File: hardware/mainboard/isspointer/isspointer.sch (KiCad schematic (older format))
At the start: 107 parts, among them J1 USB_B_Micro, J2 Motor 1, J3 Motor 2, Q1 SS8050-G, Q2 SS8050-G, Q3 DMN67D8L, Q4 DMN67D8L, SW1 Boot, SW2 Reset, SW3 Up, SW4 Select, SW5 Down, U1 AMS1117-3.3, U2 CP2102N-A01-GQFN28, U3 esp32-WROOM-32D, U4 DRV8834_HTSSOP, U5 DRV8834_HTSSOP, U6 LSM303DLHC, U7 EE-SX3350, U8 EE-SX3350, U9 CFAL12864N

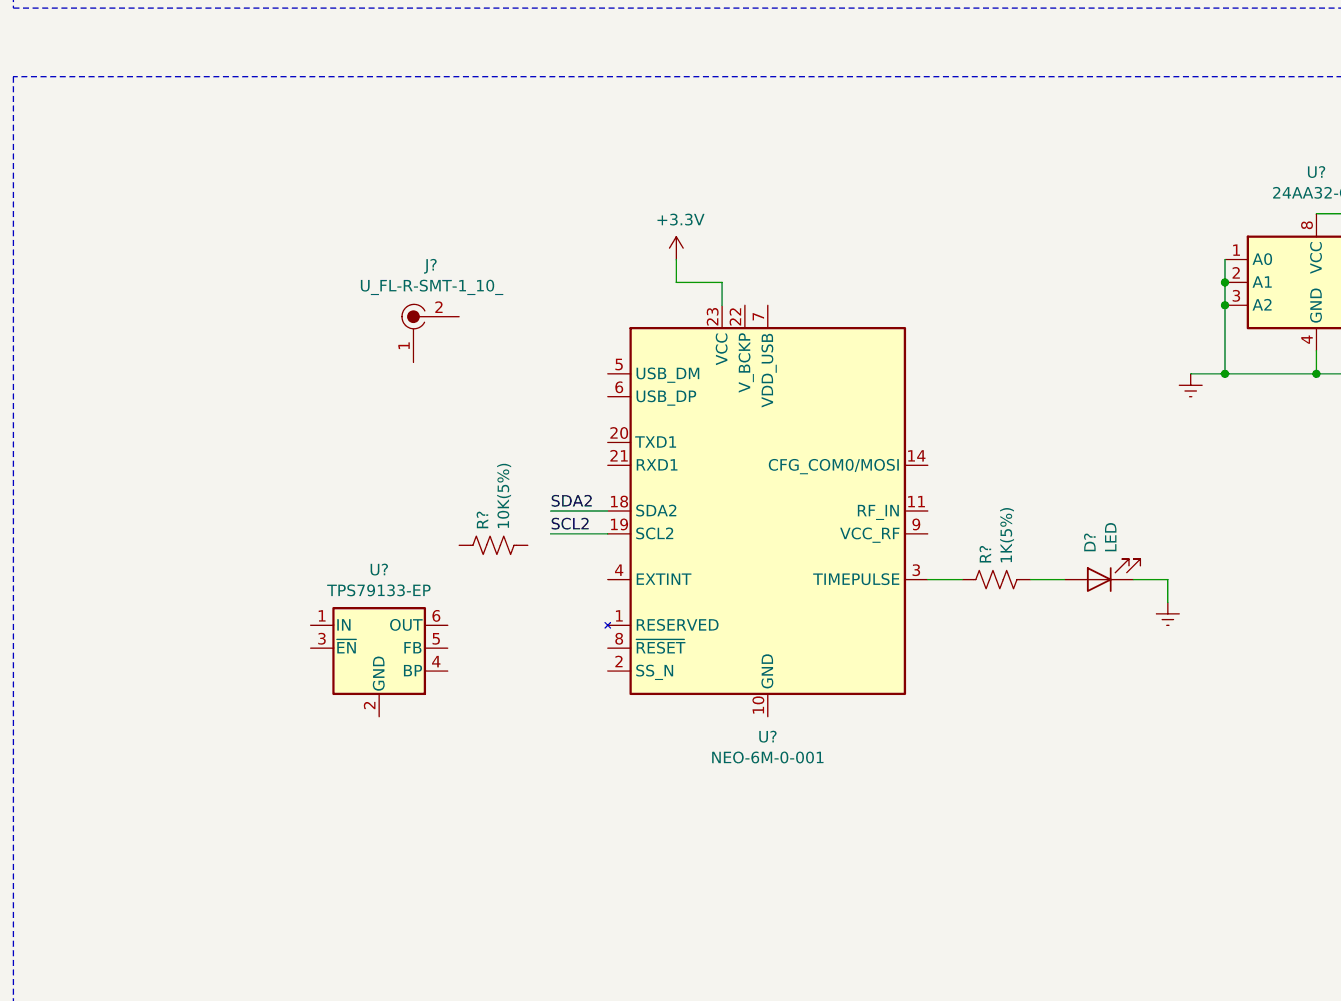
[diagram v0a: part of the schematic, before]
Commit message: minor
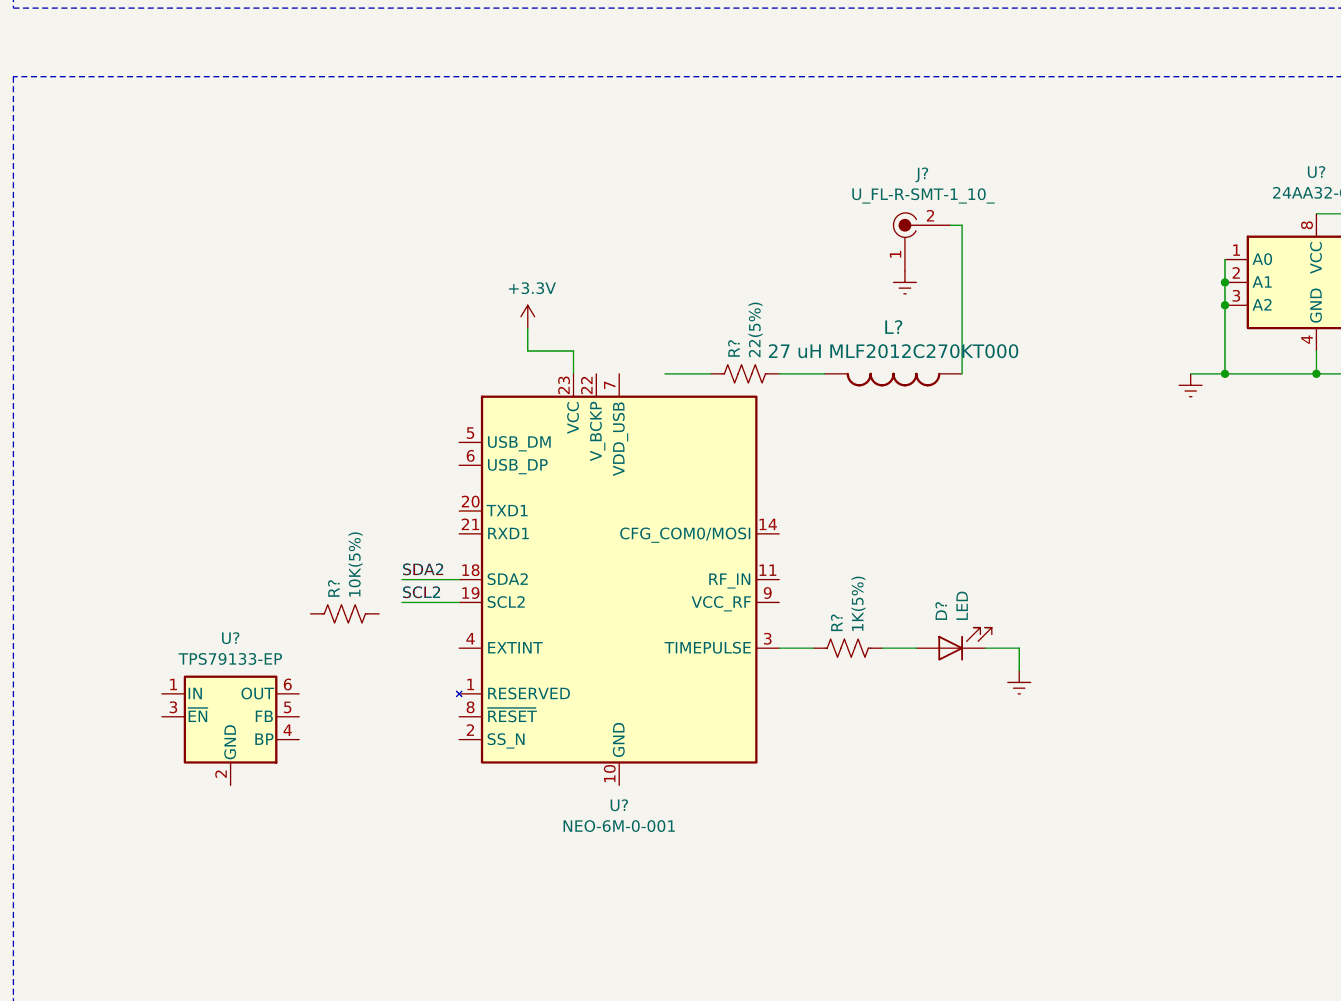
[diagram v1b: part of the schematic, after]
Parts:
- added L?: 27 uH MLF2012C270KT000, symbol isspointer-eagle-import:INDUCTOR0805
- added R?: 22(5%), Resistor_SMD:R_0603_1608Metric_Pad1.05x0.95mm_HandSolder, symbol Device:R_US
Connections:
- net GNDREF: now also J?.1
- net at J?.2: now also L?.1
- new net: L?.2, R?.1
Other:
- moved on the sheet: D?, J?, R?, U?
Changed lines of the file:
@@
 L isspointer:NEO-6M-0-001 U?
 U 1 1 5E5771B3
-P 10650 11800
-F 0 "U?" H 10650 10811 50  0000 C CNN
-F 1 "NEO-6M-0-001" H 10650 10720 50  0000 C CNN
-F 2 "RF_GPS:ublox_NEO" H 11050 10950 50  0001 C CNN
-F 3 "https://www.u-blox.com/sites/default/files/NEO-M8-FW3_DataSheet_%28UBX-15031086%29.pdf" H 10650 11800 50  0001 C CNN
-	1    10650 11800
+P 10000 12100
+F 0 "U?" H 10000 11111 50  0000 C CNN
+F 1 "NEO-6M-0-001" H 10000 11020 50  0000 C CNN
+F 2 "RF_GPS:ublox_NEO" H 10400 11250 50  0001 C CNN
+F 3 "https://www.u-blox.com/sites/default/files/NEO-M8-FW3_DataSheet_%28UBX-15031086%29.pdf" H 10000 12100 50  0001 C CNN
+	1    10000 12100
 	1    0    0    -1
 $EndComp
@@
 L isspointer:TPS79133-EP U?
 U 1 1 5E552781
-P 8950 12400
-F 0 "U?" H 8950 12742 50  0000 C CNN
-F 1 "TPS79133-EP" H 8950 12651 50  0000 C CNN
-F 2 "Package_TO_SOT_SMD:SOT-23-6" H 8950 12725 50  0001 C CIN
-F 3 "http://www.ti.com/lit/ds/symlink/tps79333-ep.pdf" H 8950 12450 50  0001 C CNN
-	1    8950 12400
+P 8300 12700
+F 0 "U?" H 8300 13042 50  0000 C CNN
+F 1 "TPS79133-EP" H 8300 12951 50  0000 C CNN
+F 2 "Package_TO_SOT_SMD:SOT-23-6" H 8300 13025 50  0001 C CIN
+F 3 "http://www.ti.com/lit/ds/symlink/tps79333-ep.pdf" H 8300 12750 50  0001 C CNN
+	1    8300 12700
 	1    0    0    -1
 $EndComp
@@
 	1    0    0    -1
 $EndComp
-Text Label 9700 11800 0    50   ~ 0
+Text Label 9050 12100 0    50   ~ 0
 SDA2
-Text Label 9700 11900 0    50   ~ 0
+Text Label 9050 12200 0    50   ~ 0
 SCL2
 Wire Wire Line
-	9950 11800 9700 11800
-Wire Wire Line
-	9950 11900 9700 11900
+	9300 12100 9050 12100
+Wire Wire Line
+	9300 12200 9050 12200
 Text Label 13700 10700 2    50   ~ 0
 SDA2
@@
 L dk_Coaxial-Connectors-RF:U_FL-R-SMT-1_10_ J?
 U 1 1 5E7CAB51
-P 9100 10950
-F 0 "J?" H 9178 11175 50  0000 C CNN
-F 1 "U_FL-R-SMT-1_10_" H 9178 11084 50  0000 C CNN
-F 2 "digikey-footprints:Coax_Conn_U.FL" H 9300 11150 60  0001 L CNN
-F 3 "https://www.hirose.com/product/en/download_file/key_name/U.FL-R-SMT-1%2810%29/category/Drawing%20(2D)/doc_file_id/37627/?file_category_id=6&item_id=03310472210&is_series=U.FL-R-SMT-1(10" H 9300 11250 60  0001 L CNN
-F 4 "H11891CT-ND" H 9300 11350 60  0001 L CNN "Digi-Key_PN"
-F 5 "U.FL-R-SMT-1(10)" H 9300 11450 60  0001 L CNN "MPN"
-F 6 "Connectors, Interconnects" H 9300 11550 60  0001 L CNN "Category"
-F 7 "Coaxial Connectors (RF)" H 9300 11650 60  0001 L CNN "Family"
-F 8 "https://www.hirose.com/product/en/download_file/key_name/U.FL-R-SMT-1%2810%29/category/Drawing%20(2D)/doc_file_id/37627/?file_category_id=6&item_id=03310472210&is_series=U.FL-R-SMT-1(10" H 9300 11750 60  0001 L CNN "DK_Datasheet_Link"
-F 9 "/product-detail/en/hirose-electric-co-ltd/U.FL-R-SMT-1(10)/H11891CT-ND/2504612" H 9300 11850 60  0001 L CNN "DK_Detail_Page"
-F 10 "CONN U.FL RCPT STR 50 OHM SMD" H 9300 11950 60  0001 L CNN "Description"
-F 11 "Hirose Electric Co Ltd" H 9300 12050 60  0001 L CNN "Manufacturer"
-F 12 "Active" H 9300 12150 60  0001 L CNN "Status"
-	1    9100 10950
+P 11250 10550
+F 0 "J?" H 11328 10775 50  0000 C CNN
+F 1 "U_FL-R-SMT-1_10_" H 11328 10684 50  0000 C CNN
+F 2 "digikey-footprints:Coax_Conn_U.FL" H 11450 10750 60  0001 L CNN
+F 3 "https://www.hirose.com/product/en/download_file/key_name/U.FL-R-SMT-1%2810%29/category/Drawing%20(2D)/doc_file_id/37627/?file_category_id=6&item_id=03310472210&is_series=U.FL-R-SMT-1(10" H 11450 10850 60  0001 L CNN
+F 4 "H11891CT-ND" H 11450 10950 60  0001 L CNN "Digi-Key_PN"
+F 5 "U.FL-R-SMT-1(10)" H 11450 11050 60  0001 L CNN "MPN"
+F 6 "Connectors, Interconnects" H 11450 11150 60  0001 L CNN "Category"
+F 7 "Coaxial Connectors (RF)" H 11450 11250 60  0001 L CNN "Family"
+F 8 "https://www.hirose.com/product/en/download_file/key_name/U.FL-R-SMT-1%2810%29/category/Drawing%20(2D)/doc_file_id/37627/?file_category_id=6&item_id=03310472210&is_series=U.FL-R-SMT-1(10" H 11450 11350 60  0001 L CNN "DK_Datasheet_Link"
+F 9 "/product-detail/en/hirose-electric-co-ltd/U.FL-R-SMT-1(10)/H11891CT-ND/2504612" H 11450 11450 60  0001 L CNN "DK_Detail_Page"
+F 10 "CONN U.FL RCPT STR 50 OHM SMD" H 11450 11550 60  0001 L CNN "Description"
+F 11 "Hirose Electric Co Ltd" H 11450 11650 60  0001 L CNN "Manufacturer"
+F 12 "Active" H 11450 11750 60  0001 L CNN "Status"
+	1    11250 10550
 	1    0    0    -1
 $EndComp
@@
 L Device:R_US R?
 U 1 1 5E7CC5CF
-P 9450 11950
-F 0 "R?" H 9382 11904 50  0000 R CNN
-F 1 "10K(5%)" H 9382 11995 50  0000 R CNN
-F 2 "Resistor_SMD:R_0603_1608Metric_Pad1.05x0.95mm_HandSolder" V 9490 11940 50  0001 C CNN
-F 3 "~" H 9450 11950 50  0001 C CNN
-	1    9450 11950
+P 8800 12250
+F 0 "R?" H 8732 12204 50  0000 R CNN
+F 1 "10K(5%)" H 8732 12295 50  0000 R CNN
+F 2 "Resistor_SMD:R_0603_1608Metric_Pad1.05x0.95mm_HandSolder" V 8840 12240 50  0001 C CNN
+F 3 "~" H 8800 12250 50  0001 C CNN
+	1    8800 12250
 	0    1    1    0
 $EndComp
@@
 L power:+3.3V #PWR?
 U 1 1 5E7F5B7C
-P 10250 10700
-F 0 "#PWR?" H 10250 10550 50  0001 C CNN
-F 1 "+3.3V" H 10267 10873 50  0000 C CNN
-F 2 "" H 10250 10700 50  0001 C CNN
-F 3 "" H 10250 10700 50  0001 C CNN
-	1    10250 10700
-	1    0    0    -1
-$EndComp
-Wire Wire Line
-	10450 10900 10450 10800
-Wire Wire Line
-	10450 10800 10250 10800
-Wire Wire Line
-	10250 10800 10250 10700
+P 9600 11000
+F 0 "#PWR?" H 9600 10850 50  0001 C CNN
+F 1 "+3.3V" H 9617 11173 50  0000 C CNN
+F 2 "" H 9600 11000 50  0001 C CNN
+F 3 "" H 9600 11000 50  0001 C CNN
+	1    9600 11000
+	1    0    0    -1
+$EndComp
+Wire Wire Line
+	9800 11200 9800 11100
+Wire Wire Line
+	9800 11100 9600 11100
+Wire Wire Line
+	9600 11100 9600 11000
 $Comp
 L Device:R_US R?
 U 1 1 5E81CF2E
-P 11650 12100
-F 0 "R?" H 11582 12054 50  0000 R CNN
-F 1 "1K(5%)" H 11582 12145 50  0000 R CNN
-F 2 "Resistor_SMD:R_0603_1608Metric_Pad1.05x0.95mm_HandSolder" V 11690 12090 50  0001 C CNN
-F 3 "~" H 11650 12100 50  0001 C CNN
-	1    11650 12100
+P 11000 12400
+F 0 "R?" H 10932 12354 50  0000 R CNN
+F 1 "1K(5%)" H 10932 12445 50  0000 R CNN
+F 2 "Resistor_SMD:R_0603_1608Metric_Pad1.05x0.95mm_HandSolder" V 11040 12390 50  0001 C CNN
+F 3 "~" H 11000 12400 50  0001 C CNN
+	1    11000 12400
 	0    1    1    0
 $EndComp
@@
 L Device:LED D?
 U 1 1 5E81DA44
-P 12100 12100
-F 0 "D?" V 12139 11983 50  0000 R CNN
-F 1 "LED" V 12048 11983 50  0000 R CNN
-F 2 "Diode_SMD:D_0603_1608Metric" H 12100 12100 50  0001 C CNN
-F 3 "~" H 12100 12100 50  0001 C CNN
-	1    12100 12100
+P 11450 12400
+F 0 "D?" V 11489 12283 50  0000 R CNN
+F 1 "LED" V 11398 12283 50  0000 R CNN
+F 2 "Diode_SMD:D_0603_1608Metric" H 11450 12400 50  0001 C CNN
+F 3 "~" H 11450 12400 50  0001 C CNN
+	1    11450 12400
 	-1   0    0    1
 $EndComp
@@
 L power:GNDREF #PWR?
 U 1 1 5E81F476
-P 12400 12200
-F 0 "#PWR?" H 12400 11950 50  0001 C CNN
-F 1 "GNDREF" H 12405 12027 50  0001 C CNN
-F 2 "" H 12400 12200 50  0001 C CNN
-F 3 "" H 12400 12200 50  0001 C CNN
-	1    12400 12200
-	1    0    0    -1
-$EndComp
-Wire Wire Line
-	11350 12100 11500 12100
-Wire Wire Line
-	11800 12100 11950 12100
-Wire Wire Line
-	12250 12100 12400 12100
-Wire Wire Line
-	12400 12100 12400 12200
+P 11750 12500
+F 0 "#PWR?" H 11750 12250 50  0001 C CNN
+F 1 "GNDREF" H 11755 12327 50  0001 C CNN
+F 2 "" H 11750 12500 50  0001 C CNN
+F 3 "" H 11750 12500 50  0001 C CNN
+	1    11750 12500
+	1    0    0    -1
+$EndComp
+Wire Wire Line
+	10700 12400 10850 12400
+Wire Wire Line
+	11150 12400 11300 12400
+Wire Wire Line
+	11600 12400 11750 12400
+Wire Wire Line
+	11750 12400 11750 12500
 $Comp
 L Device:Battery_Cell BT?
@@
 	1    0    0    -1
 $EndComp
+$Comp
+L isspointer-eagle-import:INDUCTOR0805 L?
+U 1 1 5E55D339
+P 11200 11200
+F 0 "L?" V 10998 11200 59  0000 C CNN
+F 1 "27 uH MLF2012C270KT000 " V 11103 11200 59  0000 C CNN
+F 2 "" H 11200 11200 50  0001 C CNN
+F 3 "" H 11200 11200 50  0001 C CNN
+	1    11200 11200
+	0    1    1    0
+$EndComp
+$Comp
+L Device:R_US R?
+U 1 1 5E55ED90
+P 10550 11200
+F 0 "R?" H 10482 11154 50  0000 R CNN
+F 1 "22(5%)" H 10482 11245 50  0000 R CNN
+F 2 "Resistor_SMD:R_0603_1608Metric_Pad1.05x0.95mm_HandSolder" V 10590 11190 50  0001 C CNN
+F 3 "~" H 10550 11200 50  0001 C CNN
+	1    10550 11200
+	0    1    1    0
+$EndComp
+Wire Wire Line
+	10200 11200 10400 11200
+Wire Wire Line
+	10700 11200 10900 11200
+Wire Wire Line
+	11500 11200 11500 10550
+Wire Wire Line
+	11500 10550 11450 10550
+$Comp
+L power:GNDREF #PWR?
+U 1 1 5E60C9CA
+P 11250 10750
+F 0 "#PWR?" H 11250 10500 50  0001 C CNN
+F 1 "GNDREF" H 11255 10577 50  0001 C CNN
+F 2 "" H 11250 10750 50  0001 C CNN
+F 3 "" H 11250 10750 50  0001 C CNN
+	1    11250 10750
+	1    0    0    -1
+$EndComp
